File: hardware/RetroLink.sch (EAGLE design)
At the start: 16 parts, among them U1 CH559L, U2 SN74LVC8T245PWR

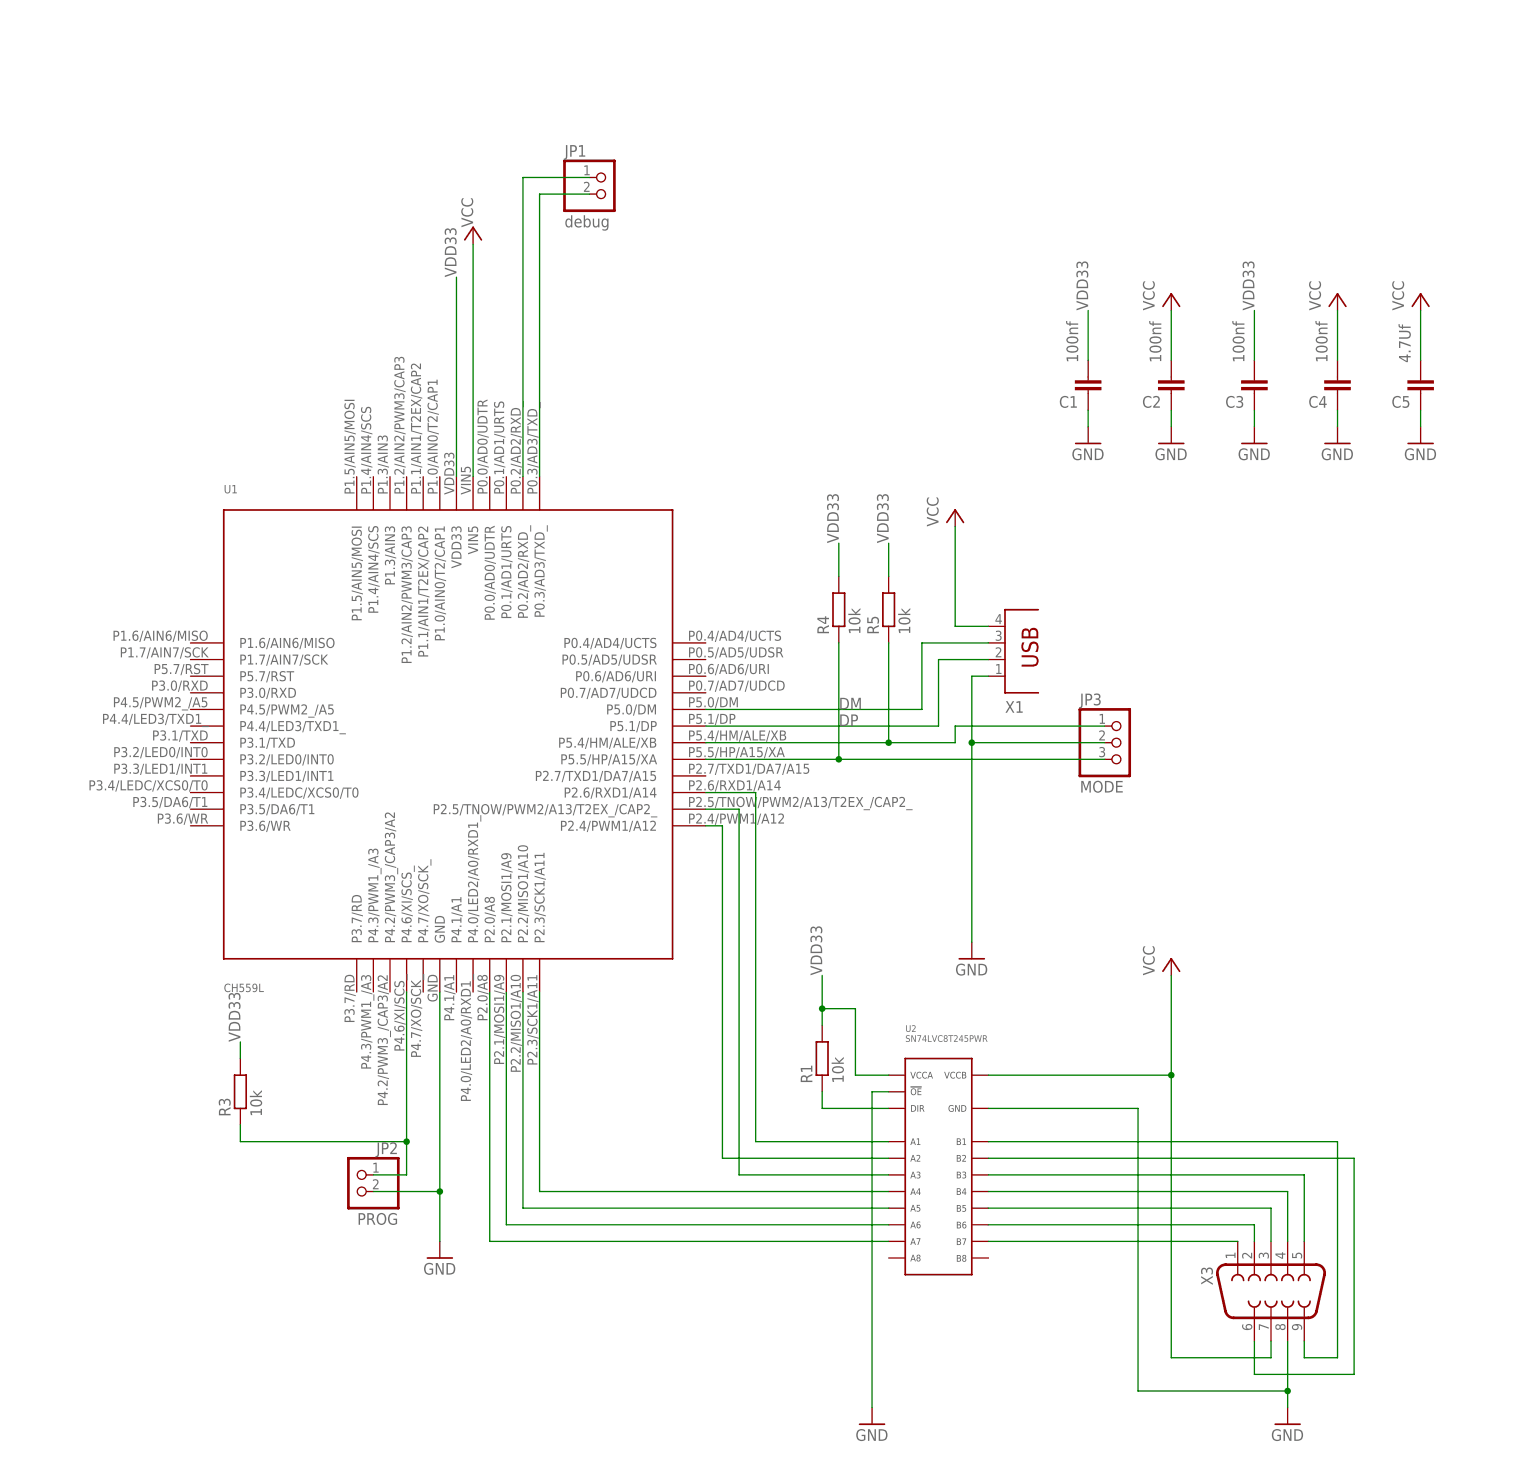
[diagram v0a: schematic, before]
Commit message: hardware and readme
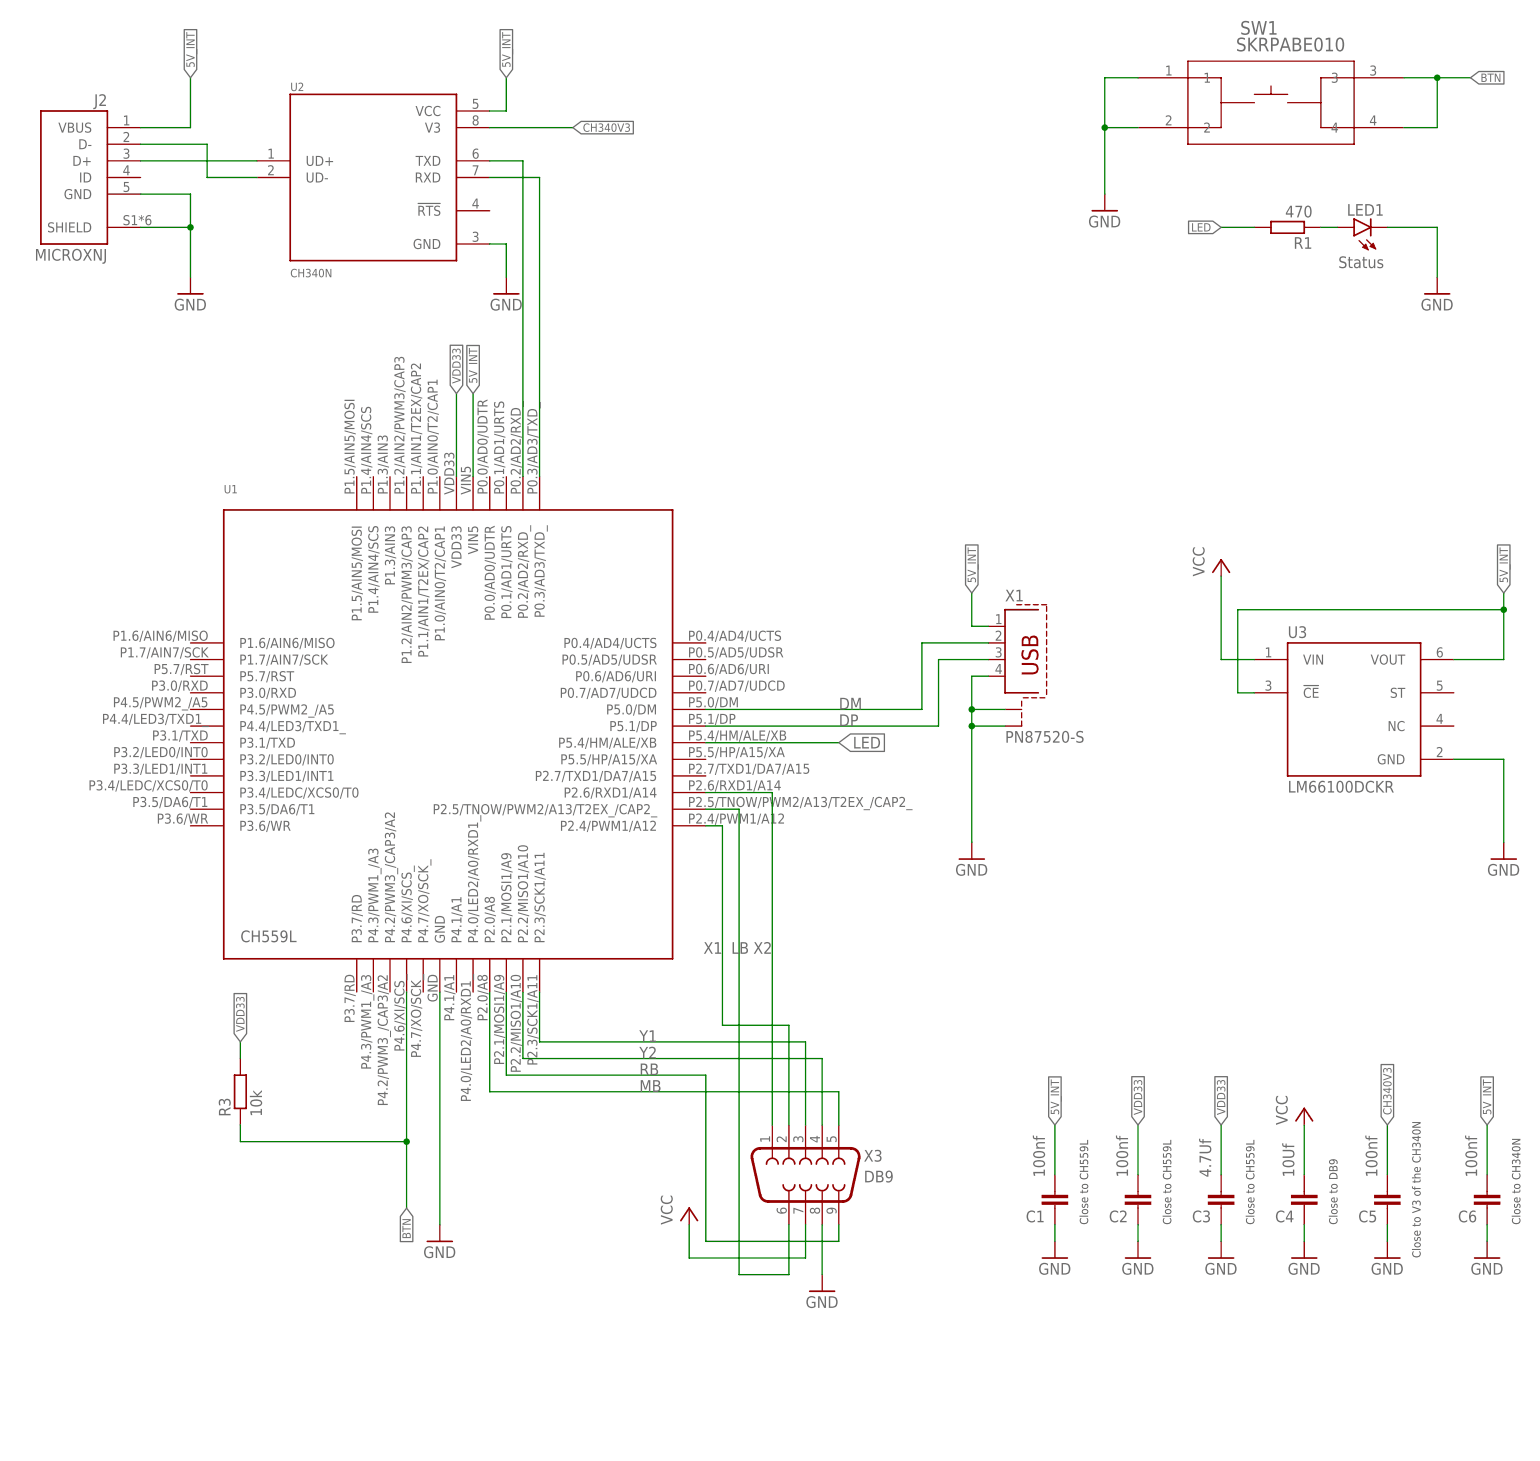
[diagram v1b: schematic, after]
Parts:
- removed JP1: debug, pinhead:PINHD-1X2
- removed JP2: PROG, pinhead:PINHD-1X2
- removed JP3: MODE, pinhead:PINHD-1X3
- removed R4, R5: 10k, rcl:R-EU_R0603
- added C6: 100nf, rcl:C-EUC0603
- added J2: MICROXNJ, MICROXNJ:MICROXNJ
- added LED1: Status, led:LEDSML0603
- added SW1: SKRPABE010, switch:SKRPABE010
- added U3: LM66100DCKR, LM66100DCKR:LM66100DCKR
- C3: value 100nf -> 4.7Uf
- C4: value 100nf -> 10Uf
- C5: value 4.7Uf -> 100nf
- R1: value 10k -> 470
- U2: value SN74LVC8T245PWR -> CH340N; device SN74LVC8T245:SN74LVC8T245PWR -> CH340N:CH340N
- X1: value (none) -> PN87520-S; device con-berg:PN87520 -> con-berg:PN87520-S
- X3: value (none) -> DB9
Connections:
- removed net N$1: U2.B7, X3.1
- removed net N$10: R1.1, U2.DIR
- removed net N$2: U2.B2, X3.6
- removed net N$3: U2.B1, X3.9
- removed net P2.0: U1.P2.0/A8, U2.A7
- removed net P2.1: U1.P2.1/MOSI1/A9, U2.A6
- removed net P2.2: U1.P2.2/MISO1/A10, U2.A5
- removed net P2.3: U1.P2.3/SCK1/A11, U2.A4
- removed net P2.4: U1.P2.4/PWM1/A12, U2.A2
- removed net P2.5: U1.P2.5/TNOW/PWM2/A13/T2EX_/CAP2_, U2.A3
- removed net P2.6: U1.P2.6/RXD1/A14, U2.A1
- removed net PROG: JP2.1, R3.1, U1.P4.6/XI/SCS_
- new net 5V_INT: C1.2, C6.2, J2.VBUS, U1.VIN5, U2.VCC, U3.!CE, U3.VOUT, X1.1
- new net BTN: R3.1, SW1.3, SW1.4, U1.P4.6/XI/SCS_
- new net CH340V3: C5.2, U2.V3
- new net LED: R1.2, U1.P5.4/HM/ALE/XB
- new net MB: U1.P2.0/A8, X3.5
- new net VLED: LED1.A, R1.1
- new net X1: U1.P2.4/PWM1/A12, X3.2
- new net X2: U1.P2.6/RXD1/A14, X3.1
- net DM: now also X1.2; no longer X1.3
- net DP: now also X1.3; no longer X1.2
- net GND: now also C6.1, J2.GND, J2.SHIELD, LED1.C, SW1.1, SW1.2, U3.GND, X1.4, X1.S1, X1.S2; no longer JP2.2, JP3.2, U2.!OE, X1.1
- net LB: now also U1.P2.5/TNOW/PWM2/A13/T2EX_/CAP2_, X3.6; no longer U2.B5, X3.3
- net N$5: now also J2.D-, U2.UD-; no longer JP3.1, R5.1, U1.P5.4/HM/ALE/XB
- net N$6: now also J2.D+, U2.UD+; no longer JP3.3, R4.1, U1.P5.5/HP/A15/XA
- net RB: now also U1.P2.1/MOSI1/A9, X3.9; no longer U2.B6, X3.2
- net RXD: now also U2.TXD; no longer JP1.1
- net TXD: now also U2.RXD; no longer JP1.2
- net VCC: now also U3.VIN; no longer C2.2, C5.2, U1.VIN5, U2.VCCB, X1.4
- net VDD33: now also C2.2; no longer C1.2, R1.2, R4.2, R5.2, U2.VCCA
- net Y1: now also U1.P2.3/SCK1/A11, X3.3; no longer U2.B3, X3.5
- net Y2: now also U1.P2.2/MISO1/A10; no longer U2.B4
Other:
- note added: "Close to CH340N"
- note added: "Close to CH559L"
- note added: "Close to DB9"
- note added: "Close to V3 of the CH340N"
- moved on the sheet: C1, C2, C3, C4, C5, R1, X3

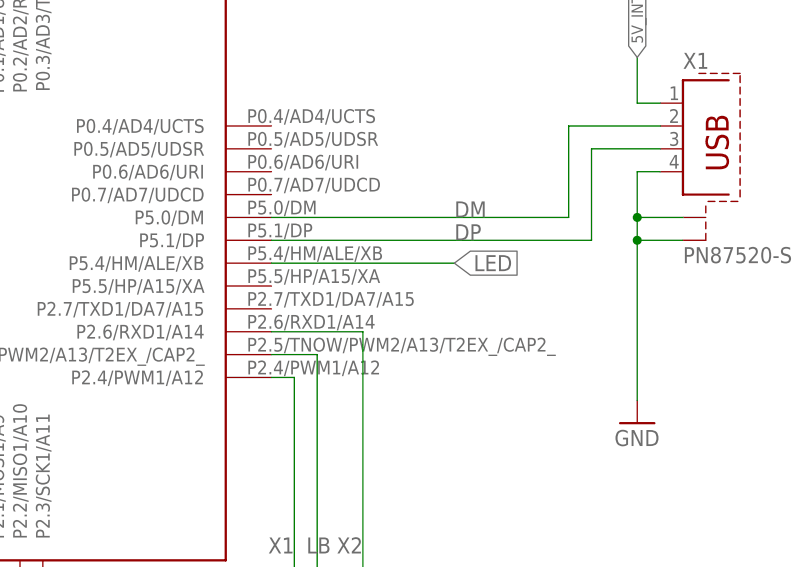
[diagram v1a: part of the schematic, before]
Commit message: led connection
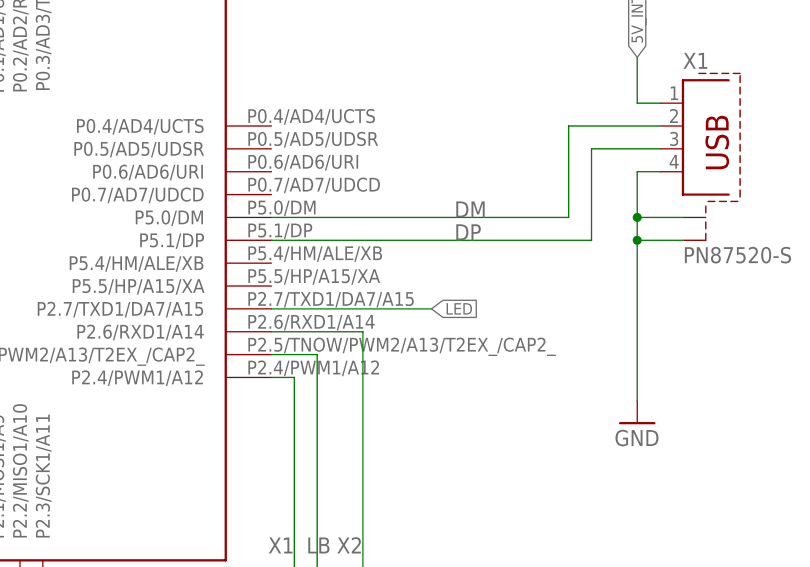
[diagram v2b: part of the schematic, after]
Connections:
- net LED: now also U1.P2.7/TXD1/DA7/A15; no longer U1.P5.4/HM/ALE/XB
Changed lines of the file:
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@@
 <segment>
 <wire x1="119.38" y1="-27.94" x2="119.38" y2="-30.48" width="0.1524" layer="91"/>
-<wire x1="119.38" y1="-30.48" x2="99.06" y2="-30.48" width="0.1524" layer="91" grouprefs="DB9"/>
+<wire x1="119.38" y1="-30.48" x2="99.06" y2="-30.48" width="0.1524" layer="91"/>
 <wire x1="99.06" y1="-30.48" x2="99.06" y2="-5.08" width="0.1524" layer="91"/>
 <wire x1="99.06" y1="-5.08" x2="68.58" y2="-5.08" width="0.1524" layer="91"/>
@@
 <segment>
 <wire x1="104.14" y1="35.56" x2="104.14" y2="-35.56" width="0.1524" layer="91"/>
-<wire x1="104.14" y1="-35.56" x2="111.76" y2="-35.56" width="0.1524" layer="91" grouprefs="DB9"/>
+<wire x1="104.14" y1="-35.56" x2="111.76" y2="-35.56" width="0.1524" layer="91"/>
 <wire x1="111.76" y1="-35.56" x2="111.76" y2="-27.94" width="0.1524" layer="91"/>
 <pinref part="X3" gate="G$1" pin="6"/>
@@
 <net name="LED" class="0">
 <segment>
-<pinref part="U1" gate="G$1" pin="P5.4/HM/ALE/XB"/>
-<wire x1="99.06" y1="45.72" x2="119.38" y2="45.72" width="0.1524" layer="91"/>
-<label x="119.38" y="45.72" size="1.778" layer="95" xref="yes"/>
-</segment>
-<segment>
 <pinref part="R1" gate="G$1" pin="2"/>
 <wire x1="182.88" y1="124.46" x2="177.8" y2="124.46" width="0.1524" layer="91" grouprefs="BUTTON_AND_LED"/>
 <label x="177.8" y="124.46" size="1.27" layer="95" rot="R180" xref="yes" grouprefs="BUTTON_AND_LED"/>
 </segment>
+<segment>
+<pinref part="U1" gate="G$1" pin="P2.7/TXD1/DA7/A15"/>
+<wire x1="99.06" y1="40.64" x2="116.84" y2="40.64" width="0.1524" layer="91"/>
+<label x="116.84" y="40.64" size="1.27" layer="95" xref="yes"/>
+</segment>
 </net>
